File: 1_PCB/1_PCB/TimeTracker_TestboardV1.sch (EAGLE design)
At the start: 24 parts, among them IC1 7805DT, IC2 7805DT, J1 2908-05WB-MG, U1 WS2812B, U2 WS2812B, U3 WS2812B, U4 WS2812B, U5 SMTM1225, Y1 FX135A-327

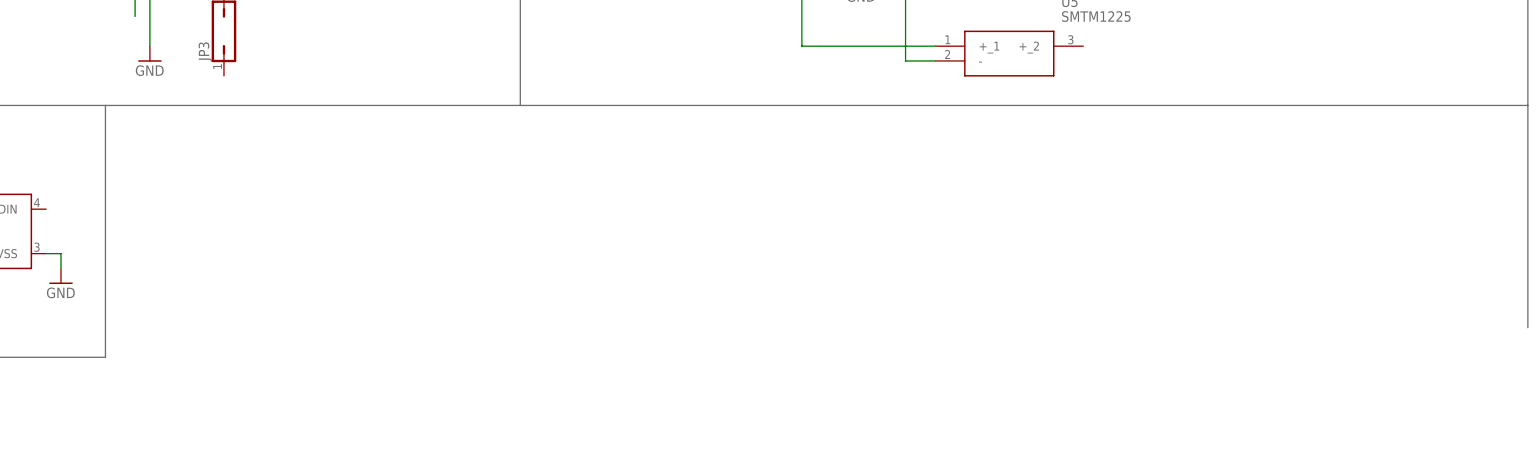
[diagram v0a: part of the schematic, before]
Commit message: Humidity and Temp Sensor
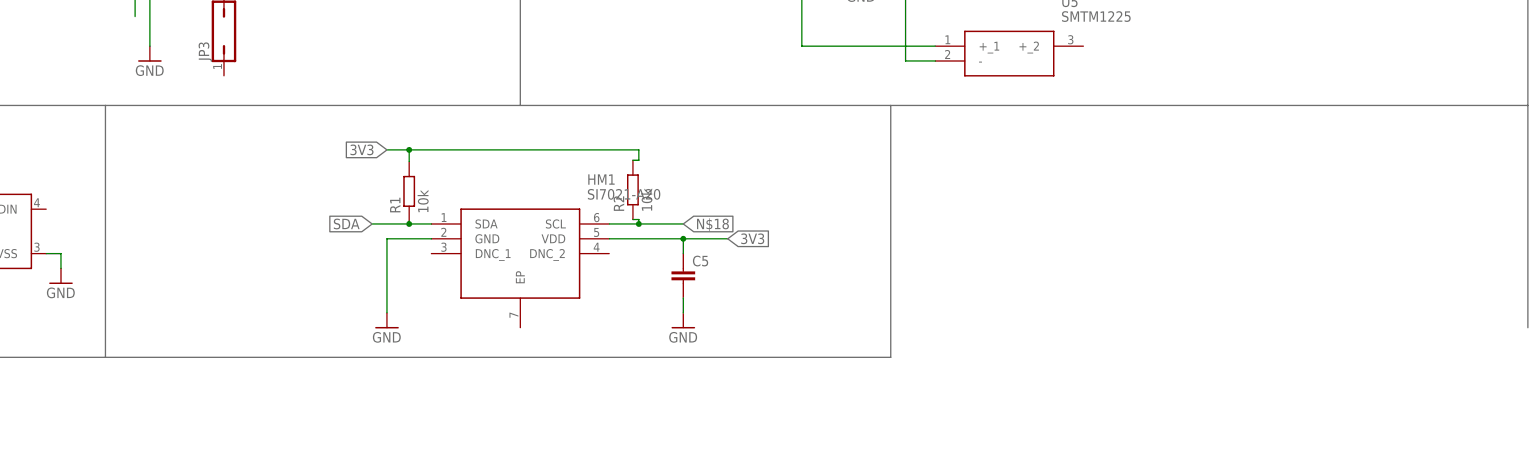
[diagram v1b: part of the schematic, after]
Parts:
- added C5: (no value), rcl:C-EUC0805
- added HM1: SI7021-A20, SamacSys_Parts:SI7021-A20
- added R1, R2: 10k, rcl:R-EU_R0805
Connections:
- new net N$18: HM1.SCL, R2.1
- new net SDA: HM1.SDA, R1.1
- net 3V3: now also C5.1, HM1.VDD, R1.2, R2.2
- net GND: now also C5.2, HM1.GND
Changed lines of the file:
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@@
 <part name="Y1" library="SamacSys_Parts" deviceset="FX135A-327" device=""/>
 <part name="U5" library="SamacSys_Parts" deviceset="SMTM1225" device=""/>
+<part name="HM1" library="SamacSys_Parts" deviceset="SI7021-A20" device=""/>
+<part name="C5" library="rcl" library_urn="urn:adsk.eagle:library:334" deviceset="C-EU" device="C0805" package3d_urn="urn:adsk.eagle:package:23617/2"/>
+<part name="GND13" library="supply1" library_urn="urn:adsk.eagle:library:371" deviceset="GND" device=""/>
+<part name="GND14" library="supply1" library_urn="urn:adsk.eagle:library:371" deviceset="GND" device=""/>
+<part name="R1" library="rcl" library_urn="urn:adsk.eagle:library:334" deviceset="R-EU_" device="R0805" package3d_urn="urn:adsk.eagle:package:23553/2" value="10k"/>
+<part name="R2" library="rcl" library_urn="urn:adsk.eagle:library:334" deviceset="R-EU_" device="R0805" package3d_urn="urn:adsk.eagle:package:23553/2" value="10k"/>
 </parts>
 <sheets>
@@
 <wire x1="167.64" y1="99.06" x2="167.64" y2="137.16" width="0.1524" layer="95"/>
 <wire x1="167.64" y1="137.16" x2="167.64" y2="205.74" width="0.1524" layer="95"/>
-<wire x1="167.64" y1="137.16" x2="-5.08" y2="137.16" width="0.1524" layer="95"/>
+<wire x1="167.64" y1="137.16" x2="58.42" y2="137.16" width="0.1524" layer="95"/>
+<wire x1="58.42" y1="137.16" x2="-5.08" y2="137.16" width="0.1524" layer="95"/>
 <wire x1="-236.22" y1="93.98" x2="-236.22" y2="137.16" width="0.1524" layer="95"/>
 <wire x1="-76.2" y1="93.98" x2="-236.22" y2="93.98" width="0.1524" layer="95"/>
 <wire x1="-76.2" y1="137.16" x2="-76.2" y2="93.98" width="0.1524" layer="95"/>
+<wire x1="58.42" y1="93.98" x2="-76.2" y2="93.98" width="0.1524" layer="95"/>
+<wire x1="58.42" y1="137.16" x2="58.42" y2="93.98" width="0.1524" layer="95"/>
 </plain>
 <instances>
@@
 <attribute name="NAME" x="87.63" y="154.94" size="1.778" layer="95" align="center-left"/>
 <attribute name="VALUE" x="87.63" y="152.4" size="1.778" layer="96" align="center-left"/>
+</instance>
+<instance part="HM1" gate="G$1" x="-20.32" y="116.84" smashed="yes">
+<attribute name="NAME" x="6.35" y="124.46" size="1.778" layer="95" align="center-left"/>
+<attribute name="VALUE" x="6.35" y="121.92" size="1.778" layer="96" align="center-left"/>
+</instance>
+<instance part="C5" gate="G$1" x="22.86" y="109.22" smashed="yes">
+<attribute name="NAME" x="24.384" y="109.601" size="1.778" layer="95"/>
+<attribute name="VALUE" x="24.384" y="104.521" size="1.778" layer="96"/>
+</instance>
+<instance part="GND13" gate="1" x="-27.94" y="99.06" smashed="yes">
+<attribute name="VALUE" x="-30.48" y="96.52" size="1.778" layer="96"/>
+</instance>
+<instance part="GND14" gate="1" x="22.86" y="99.06" smashed="yes">
+<attribute name="VALUE" x="20.32" y="96.52" size="1.778" layer="96"/>
+</instance>
+<instance part="R1" gate="G$1" x="-24.13" y="122.428" smashed="yes" rot="R90">
+<attribute name="NAME" x="-25.6286" y="118.618" size="1.778" layer="95" rot="R90"/>
+<attribute name="VALUE" x="-20.828" y="118.618" size="1.778" layer="96" rot="R90"/>
+</instance>
+<instance part="R2" gate="G$1" x="14.224" y="122.682" smashed="yes" rot="R90">
+<attribute name="NAME" x="12.7254" y="118.872" size="1.778" layer="95" rot="R90"/>
+<attribute name="VALUE" x="17.526" y="118.872" size="1.778" layer="96" rot="R90"/>
 </instance>
 </instances>
@@
 <wire x1="104.14" y1="180.34" x2="116.84" y2="180.34" width="0.1524" layer="91"/>
 <label x="116.84" y="180.34" size="1.778" layer="95" xref="yes"/>
+</segment>
+<segment>
+<pinref part="HM1" gate="G$1" pin="VDD"/>
+<wire x1="10.16" y1="114.3" x2="22.86" y2="114.3" width="0.1524" layer="91"/>
+<label x="30.48" y="114.3" size="1.778" layer="95" xref="yes"/>
+<pinref part="C5" gate="G$1" pin="1"/>
+<wire x1="22.86" y1="114.3" x2="30.48" y2="114.3" width="0.1524" layer="91"/>
+<wire x1="22.86" y1="111.76" x2="22.86" y2="114.3" width="0.1524" layer="91"/>
+<junction x="22.86" y="114.3"/>
+</segment>
+<segment>
+<wire x1="-27.94" y1="129.54" x2="-24.13" y2="129.54" width="0.1524" layer="91"/>
+<pinref part="R1" gate="G$1" pin="2"/>
+<wire x1="-24.13" y1="129.54" x2="15.24" y2="129.54" width="0.1524" layer="91"/>
+<wire x1="-24.13" y1="127.508" x2="-24.13" y2="129.54" width="0.1524" layer="91"/>
+<pinref part="R2" gate="G$1" pin="2"/>
+<wire x1="14.224" y1="127.762" x2="15.24" y2="127.762" width="0.1524" layer="91"/>
+<wire x1="15.24" y1="127.762" x2="15.24" y2="129.54" width="0.1524" layer="91"/>
+<junction x="-24.13" y="129.54"/>
+<label x="-27.94" y="129.54" size="1.778" layer="95" rot="R180" xref="yes"/>
 </segment>
 </net>
@@
 <pinref part="GND36" gate="1" pin="GND"/>
 <wire x1="-200.66" y1="152.4" x2="-200.66" y2="147.32" width="0.1524" layer="91"/>
+</segment>
+<segment>
+<pinref part="HM1" gate="G$1" pin="GND"/>
+<wire x1="-20.32" y1="114.3" x2="-27.94" y2="114.3" width="0.1524" layer="91"/>
+<wire x1="-27.94" y1="114.3" x2="-27.94" y2="101.6" width="0.1524" layer="91"/>
+<pinref part="GND13" gate="1" pin="GND"/>
+</segment>
+<segment>
+<pinref part="C5" gate="G$1" pin="2"/>
+<pinref part="GND14" gate="1" pin="GND"/>
+<wire x1="22.86" y1="104.14" x2="22.86" y2="101.6" width="0.1524" layer="91"/>
 </segment>
 </net>
@@
 </segment>
 </net>
+<net name="SDA" class="0">
+<segment>
+<pinref part="HM1" gate="G$1" pin="SDA"/>
+<wire x1="-20.32" y1="116.84" x2="-24.13" y2="116.84" width="0.1524" layer="91"/>
+<label x="-30.48" y="116.84" size="1.778" layer="95" rot="R180" xref="yes"/>
+<pinref part="R1" gate="G$1" pin="1"/>
+<wire x1="-24.13" y1="116.84" x2="-30.48" y2="116.84" width="0.1524" layer="91"/>
+<wire x1="-24.13" y1="117.348" x2="-24.13" y2="116.84" width="0.1524" layer="91"/>
+<junction x="-24.13" y="116.84"/>
+<wire x1="-24.13" y1="116.84" x2="-24.13" y2="116.586" width="0.1524" layer="91"/>
+</segment>
+</net>
+<net name="N$18" class="0">
+<segment>
+<pinref part="HM1" gate="G$1" pin="SCL"/>
+<wire x1="10.16" y1="116.84" x2="15.24" y2="116.84" width="0.1524" layer="91"/>
+<label x="22.86" y="116.84" size="1.778" layer="95" xref="yes"/>
+<pinref part="R2" gate="G$1" pin="1"/>
+<wire x1="15.24" y1="116.84" x2="22.86" y2="116.84" width="0.1524" layer="91"/>
+<wire x1="14.224" y1="117.602" x2="15.24" y2="117.602" width="0.1524" layer="91"/>
+<wire x1="15.24" y1="117.602" x2="15.24" y2="116.84" width="0.1524" layer="91"/>
+<junction x="15.24" y="116.84"/>
+</segment>
+</net>
